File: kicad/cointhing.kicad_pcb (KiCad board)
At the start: 2 copper layers, 35 x 34 mm, 27 parts, among them J1 USB_B_Micro, Q1 PUMX1, Q2 S8050_J3Y, U1 ESP-12E, U2 CP2102-GMR_NRND, U3 BL8565, U4 74AHC1G08

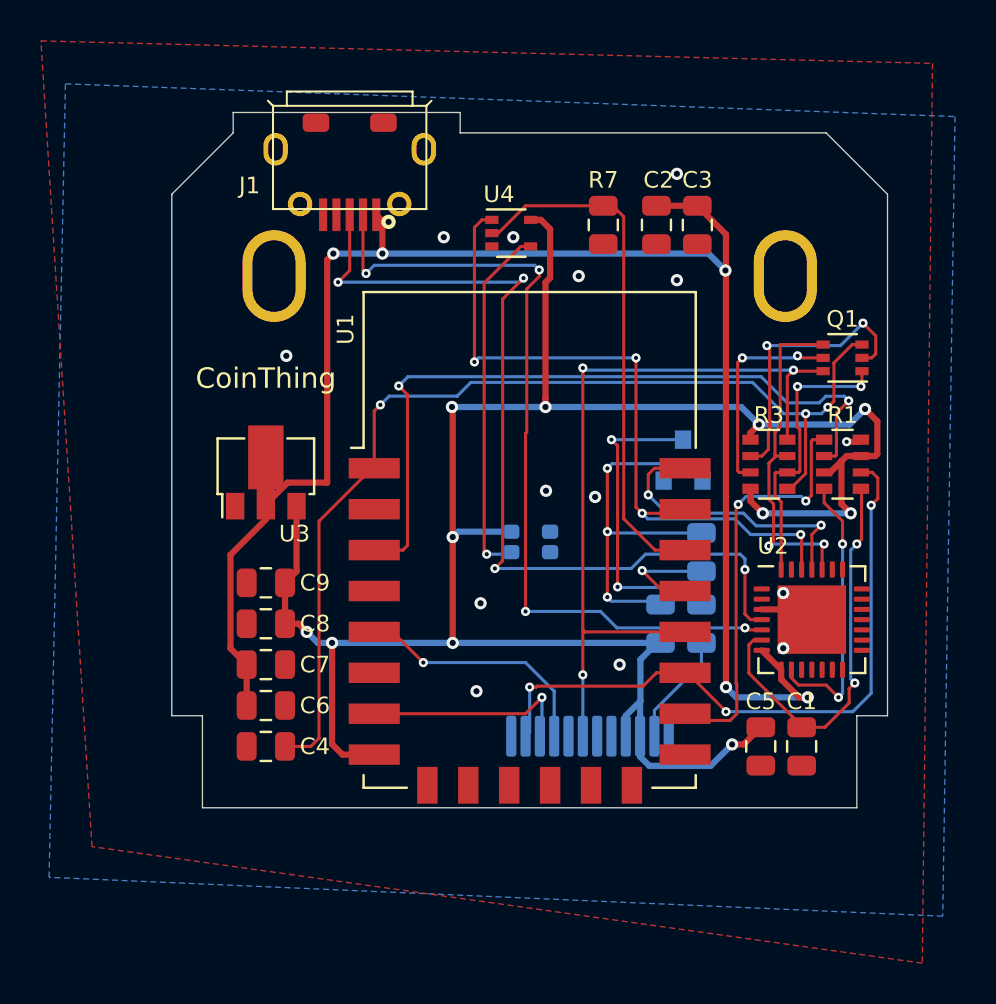
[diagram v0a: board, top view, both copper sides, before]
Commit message: changes for pcb and case
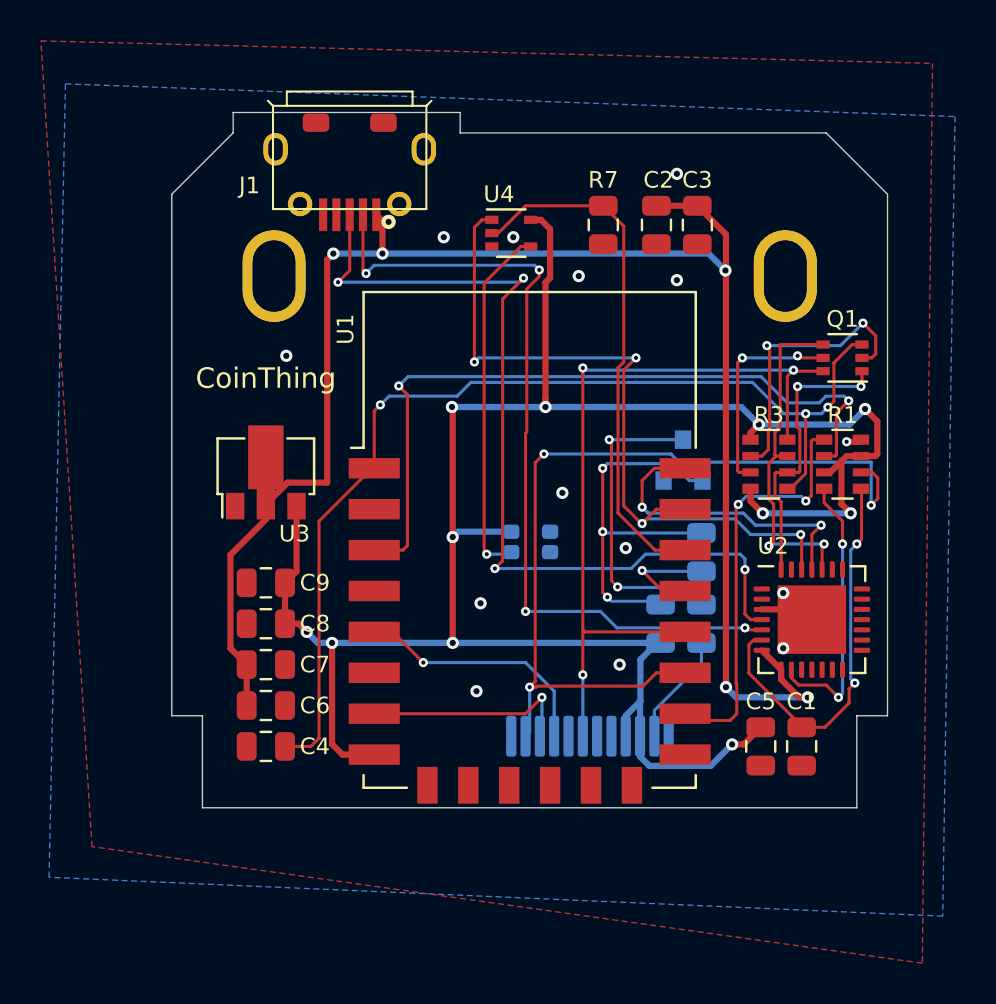
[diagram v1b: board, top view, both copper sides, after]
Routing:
- net /~TFT_RES: track 32.2 -> 42.7 mm
- net /TxD: track 35.4 -> 36.6 mm
- net /RxD: track 14.4 -> 15.1 mm
